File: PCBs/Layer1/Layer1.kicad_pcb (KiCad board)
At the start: 2 copper layers, 90 x 90 mm, 52 parts, among them J1 Screw_Terminal_01x02, J2 Conn_01x12, T1 T60404-E4624-X501, U1 STPM_STPM10BTR, U2 level_shifter, U3 Micro_SD_Shield, U4 DOIT_ESP32_Devkit_v1-MCU_Modu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, Y1 4.194304 MHz

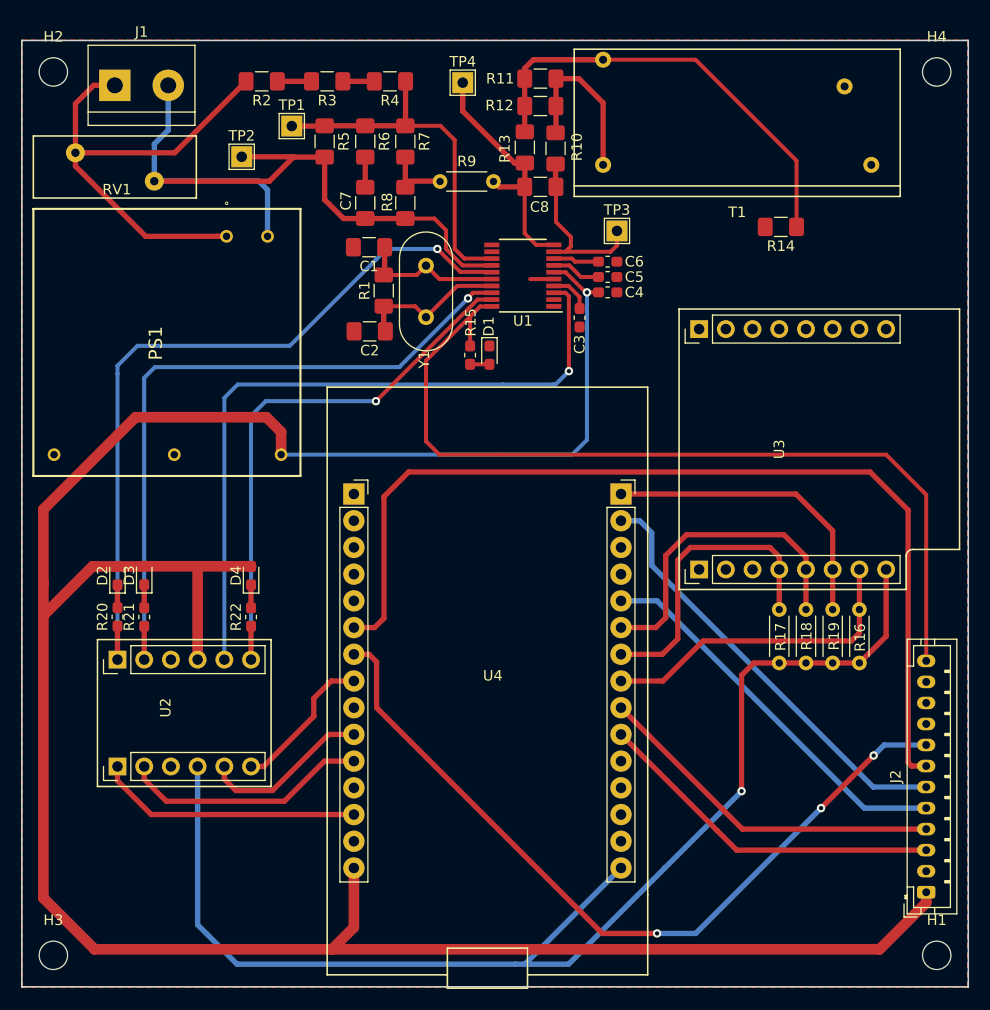
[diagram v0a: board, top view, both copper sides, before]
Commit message: WIP: version 2 schematics
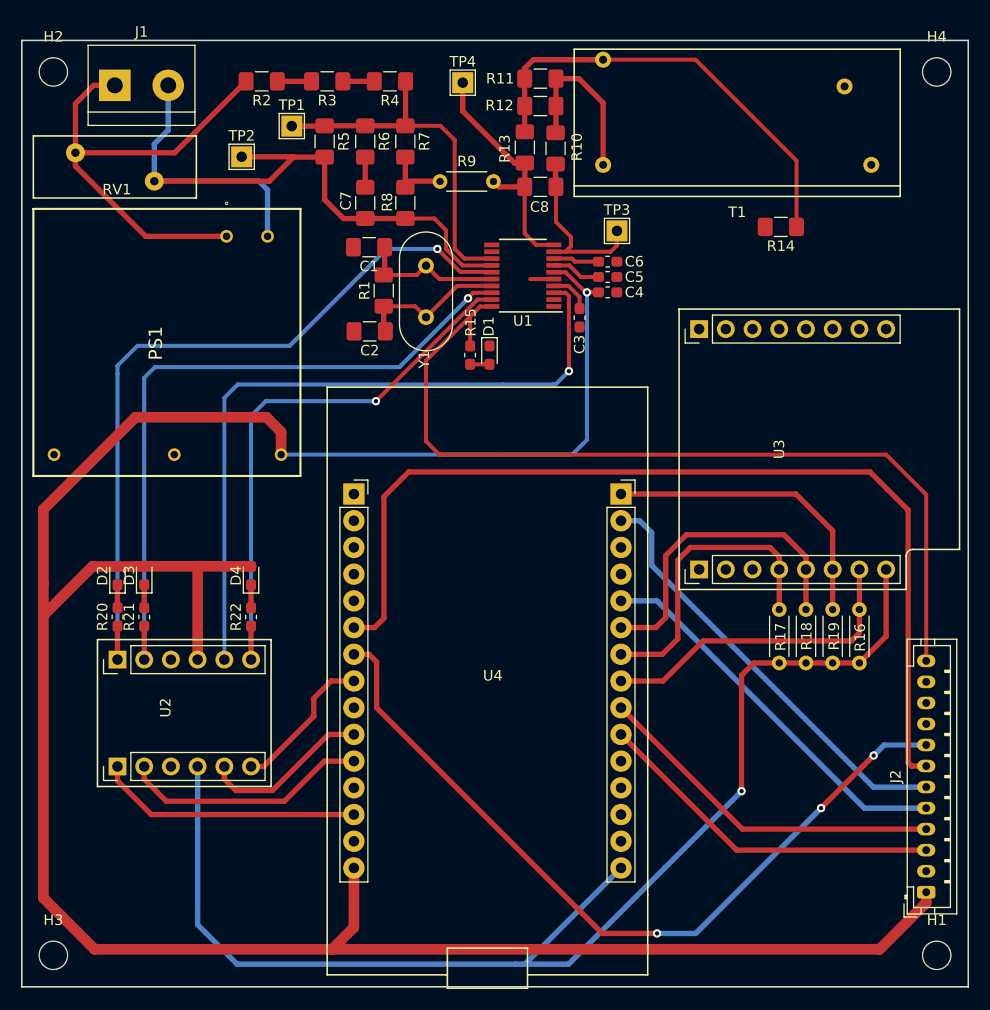
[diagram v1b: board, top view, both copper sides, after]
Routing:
- removed copper zone on F.Cu, net GND
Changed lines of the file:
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@@
   )
   (setup
-    (last_trace_width 0.381)
+    (last_trace_width 0.25)
     (user_trace_width 0.381)
     (user_trace_width 0.508)
@@
     (solder_mask_min_width 0.25)
     (aux_axis_origin 13 13)
-    (visible_elements FFFFFF7F)
+    (visible_elements FFFFF77F)
     (pcbplotparams
       (layerselection 0x010fc_ffffffff)
@@
   (segment (start 24.638 66.957) (end 24.638 64.756) (width 0.508) (layer F.Cu) (net 70))
   (segment (start 22.098 66.943) (end 22.098 64.77) (width 0.508) (layer F.Cu) (net 71))
-  (zone (net 0) (net_name "") (layer F.Cu) (hatch edge 0.508)
-    (connect_pads (clearance 0.508))
-    (min_thickness 0.254)
-    (keepout (tracks allowed) (vias allowed) (copperpour not_allowed))
-    (fill (arc_segments 16) (thermal_gap 0.508) (thermal_bridge_width 0.508))
-    (polygon
-      (pts
-        (xy 13 13) (xy 13 36) (xy 40 36) (xy 40 25) (xy 52 25)
-        (xy 52 13)
-      )
-    )
-  )
-  (zone (net 2) (net_name GND) (layer F.Cu) (hatch edge 0.508)
-    (connect_pads (clearance 0.508))
-    (min_thickness 0.254)
-    (fill (arc_segments 16) (thermal_gap 0.508) (thermal_bridge_width 0.508))
-    (polygon
-      (pts
-        (xy 13 13) (xy 103 13) (xy 103 103) (xy 13 103)
-      )
-    )
-  )
-  (zone (net 2) (net_name GND) (layer F.Cu) (hatch edge 0.508)
-    (connect_pads (clearance 0.508))
-    (min_thickness 0.254)
-    (fill (arc_segments 16) (thermal_gap 0.508) (thermal_bridge_width 0.508))
-    (polygon
-      (pts
-        (xy 13 13) (xy 103 13) (xy 103 103) (xy 13 103)
-      )
-    )
-  )
 )
